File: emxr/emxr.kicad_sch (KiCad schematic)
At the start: 13 parts, among them J101 POWER, J103 Bus Conn, J104 GEQ_L_PRE, J105 GEQ_L_POST, J106 GEQ_R_PRE, J107 GEQ_R_POST, J108 AUDIO_OUT

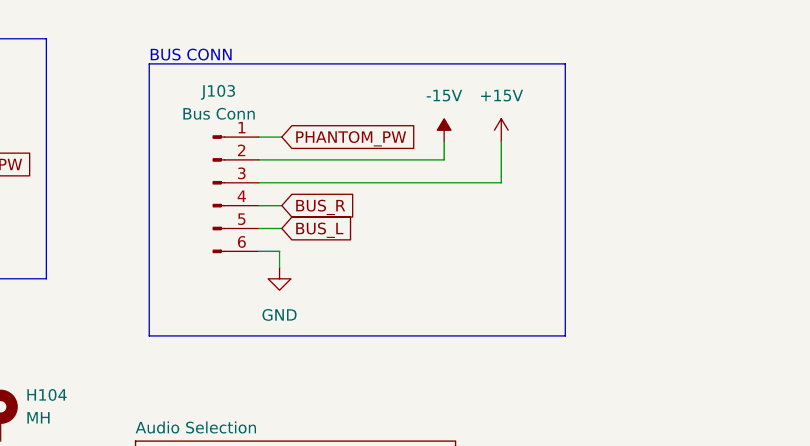
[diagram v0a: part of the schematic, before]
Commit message: finished pcb draft
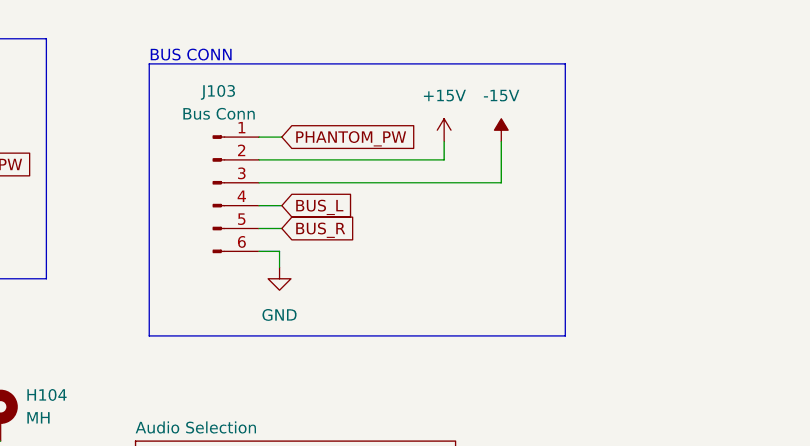
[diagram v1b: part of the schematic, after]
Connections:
- net +15V: now also J103.2 (Pin_2); no longer J103.3 (Pin_3)
- net -15V: now also J103.3 (Pin_3); no longer J103.2 (Pin_2)
- net BUS_L: now also J103.4 (Pin_4); no longer J103.5 (Pin_5)
- net BUS_R: now also J103.5 (Pin_5); no longer J103.4 (Pin_4)
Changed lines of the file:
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@@
+    )
+  )
+  (global_label "BUS_L" (shape input) (at 72.898 37.084 0) (fields_autoplaced)
+    (effects (font (size 1.27 1.27)) (justify left))
+    (property "Intersheet References" "${INTERSHEET_REFS}" (id 0) (at 81.1168 37.0046 0)
+      (effects (font (size 1.27 1.27)) (justify left) hide)
     )
   )
@@
     )
   )
-  (global_label "BUS_L" (shape input) (at 72.898 39.624 0) (fields_autoplaced)
-    (effects (font (size 1.27 1.27)) (justify left))
-    (property "Intersheet References" "${INTERSHEET_REFS}" (id 0) (at 81.1168 39.5446 0)
-      (effects (font (size 1.27 1.27)) (justify left) hide)
-    )
-  )
   (global_label "SINGAL_L_POST_GEQ" (shape input) (at 254.254 103.886 180) (fields_autoplaced)
     (effects (font (size 1.27 1.27)) (justify right))
@@
     )
   )
-  (global_label "BUS_R" (shape input) (at 72.898 37.084 0) (fields_autoplaced)
-    (effects (font (size 1.27 1.27)) (justify left))
-    (property "Intersheet References" "${INTERSHEET_REFS}" (id 0) (at 81.3587 37.0046 0)
-      (effects (font (size 1.27 1.27)) (justify left) hide)
-    )
-  )
   (global_label "SINGAL_R_PRE_GEQ" (shape input) (at 115.57 110.49 180) (fields_autoplaced)
     (effects (font (size 1.27 1.27)) (justify right))
@@
     )
   )
+  (global_label "BUS_R" (shape input) (at 72.898 39.624 0) (fields_autoplaced)
+    (effects (font (size 1.27 1.27)) (justify left))
+    (property "Intersheet References" "${INTERSHEET_REFS}" (id 0) (at 81.3587 39.5446 0)
+      (effects (font (size 1.27 1.27)) (justify left) hide)
+    )
+  )
   (symbol (lib_id "Connector:Conn_01x04_Male") (at 21.336 29.972 0) (unit 1)
     (in_bom yes) (on_board yes) (fields_autoplaced)
@@
     (pin "4")
   )
+  (symbol (lib_id "power:-15V") (at 97.282 29.972 0) (unit 1)
+    (in_bom yes) (on_board yes) (fields_autoplaced)
+    (property "Reference" "#PWR0117" (id 0) (at 97.282 27.432 0)
+      (effects (font (size 1.27 1.27)) hide)
+    )
+    (property "Value" "-15V" (id 1) (at 97.282 24.892 0))
+    (property "Footprint" "" (id 2) (at 97.282 29.972 0)
+      (effects (font (size 1.27 1.27)) hide)
+    )
+    (property "Datasheet" "" (id 3) (at 97.282 29.972 0)
+      (effects (font (size 1.27 1.27)) hide)
+    )
+    (pin "1")
+  )
   (symbol (lib_id "Mechanical:MountingHole_Pad") (at 34.036 60.706 0) (unit 1)
     (in_bom yes) (on_board yes) (fields_autoplaced)
@@
     (pin "1")
     (pin "2")
-  )
-  (symbol (lib_id "power:-15V") (at 36.576 26.162 0) (unit 1)
-    (in_bom yes) (on_board yes) (fields_autoplaced)
-    (property "Reference" "#PWR0102" (id 0) (at 36.576 23.622 0)
-      (effects (font (size 1.27 1.27)) hide)
-    )
-    (property "Value" "-15V" (id 1) (at 36.576 21.082 0))
-    (property "Footprint" "" (id 2) (at 36.576 26.162 0)
-      (effects (font (size 1.27 1.27)) hide)
-    )
-    (property "Datasheet" "" (id 3) (at 36.576 26.162 0)
-      (effects (font (size 1.27 1.27)) hide)
-    )
-    (pin "1")
   )
   (symbol (lib_id "power:GND") (at 28.956 37.592 0) (unit 1)
@@
     (pin "2")
   )
+  (symbol (lib_id "power:-15V") (at 36.576 26.162 0) (unit 1)
+    (in_bom yes) (on_board yes) (fields_autoplaced)
+    (property "Reference" "#PWR0102" (id 0) (at 36.576 23.622 0)
+      (effects (font (size 1.27 1.27)) hide)
+    )
+    (property "Value" "-15V" (id 1) (at 36.576 21.082 0))
+    (property "Footprint" "" (id 2) (at 36.576 26.162 0)
+      (effects (font (size 1.27 1.27)) hide)
+    )
+    (property "Datasheet" "" (id 3) (at 36.576 26.162 0)
+      (effects (font (size 1.27 1.27)) hide)
+    )
+    (pin "1")
+  )
   (symbol (lib_id "power:GND") (at 115.57 102.87 0) (unit 1)
     (in_bom yes) (on_board yes)
@@
     (pin "1")
   )
-  (symbol (lib_id "power:-15V") (at 90.932 29.972 0) (unit 1)
-    (in_bom yes) (on_board yes) (fields_autoplaced)
-    (property "Reference" "#PWR0117" (id 0) (at 90.932 27.432 0)
-      (effects (font (size 1.27 1.27)) hide)
-    )
-    (property "Value" "-15V" (id 1) (at 90.932 24.892 0))
-    (property "Footprint" "" (id 2) (at 90.932 29.972 0)
-      (effects (font (size 1.27 1.27)) hide)
-    )
-    (property "Datasheet" "" (id 3) (at 90.932 29.972 0)
+  (symbol (lib_id "power:+15V") (at 30.226 26.162 0) (unit 1)
+    (in_bom yes) (on_board yes) (fields_autoplaced)
+    (property "Reference" "#PWR0101" (id 0) (at 30.226 29.972 0)
+      (effects (font (size 1.27 1.27)) hide)
+    )
+    (property "Value" "+15V" (id 1) (at 30.226 21.082 0))
+    (property "Footprint" "" (id 2) (at 30.226 26.162 0)
+      (effects (font (size 1.27 1.27)) hide)
+    )
+    (property "Datasheet" "" (id 3) (at 30.226 26.162 0)
       (effects (font (size 1.27 1.27)) hide)
     )
@@
     (pin "3")
   )
+  (symbol (lib_id "power:+15V") (at 90.932 29.972 0) (unit 1)
+    (in_bom yes) (on_board yes)
+    (property "Reference" "#PWR0105" (id 0) (at 90.932 33.782 0)
+      (effects (font (size 1.27 1.27)) hide)
+    )
+    (property "Value" "+15V" (id 1) (at 90.932 24.892 0))
+    (property "Footprint" "" (id 2) (at 90.932 29.972 0)
+      (effects (font (size 1.27 1.27)) hide)
+    )
+    (property "Datasheet" "" (id 3) (at 90.932 29.972 0)
+      (effects (font (size 1.27 1.27)) hide)
+    )
+    (pin "1")
+  )
   (symbol (lib_id "Mechanical:MountingHole_Pad") (at 18.542 60.706 0) (unit 1)
     (in_bom yes) (on_board yes) (fields_autoplaced)
@@
     )
     (property "Datasheet" "~" (id 3) (at 27.94 27.432 0)
-      (effects (font (size 1.27 1.27)) hide)
-    )
-    (pin "1")
-  )
-  (symbol (lib_id "power:+15V") (at 97.282 29.972 0) (unit 1)
-    (in_bom yes) (on_board yes)
-    (property "Reference" "#PWR0105" (id 0) (at 97.282 33.782 0)
-      (effects (font (size 1.27 1.27)) hide)
-    )
-    (property "Value" "+15V" (id 1) (at 97.282 24.892 0))
-    (property "Footprint" "" (id 2) (at 97.282 29.972 0)
-      (effects (font (size 1.27 1.27)) hide)
-    )
-    (property "Datasheet" "" (id 3) (at 97.282 29.972 0)
-      (effects (font (size 1.27 1.27)) hide)
-    )
-    (pin "1")
-  )
-  (symbol (lib_id "power:+15V") (at 30.226 26.162 0) (unit 1)
-    (in_bom yes) (on_board yes) (fields_autoplaced)
-    (property "Reference" "#PWR0101" (id 0) (at 30.226 29.972 0)
-      (effects (font (size 1.27 1.27)) hide)
-    )
-    (property "Value" "+15V" (id 1) (at 30.226 21.082 0))
-    (property "Footprint" "" (id 2) (at 30.226 26.162 0)
-      (effects (font (size 1.27 1.27)) hide)
-    )
-    (property "Datasheet" "" (id 3) (at 30.226 26.162 0)
       (effects (font (size 1.27 1.27)) hide)
     )
@@
       (reference "#FLG0302") (unit 1) (value "PWR_FLAG") (footprint "")
     )
-    (path "/f7fcb284-2c50-4899-a801-6bc09b570947"
+    (path "/ca94f7d8-1a2e-4977-bdda-6569c606eee3"
       (reference "#PWR0101") (unit 1) (value "+15V") (footprint "")
     )
-    (path "/318c314c-3085-4786-b774-c74338b7a2e5"
+    (path "/969dab04-7c43-4161-8376-eb4539bfe8f0"
       (reference "#PWR0102") (unit 1) (value "-15V") (footprint "")
     )
@@
       (reference "#PWR0104") (unit 1) (value "GND") (footprint "")
     )
-    (path "/ee4aa2f5-45df-4dae-abad-1cf46d567827"
+    (path "/daf14d0e-21df-46a4-877f-4f85481a5d4a"
       (reference "#PWR0105") (unit 1) (value "+15V") (footprint "")
     )
@@
       (reference "#PWR0116") (unit 1) (value "GND") (footprint "")
     )
-    (path "/d20691b9-17e8-4af0-b9bd-2f8e4c1bd205"
+    (path "/1290aab4-682e-4097-b981-7d63f0a8b5a2"
       (reference "#PWR0117") (unit 1) (value "-15V") (footprint "")
     )

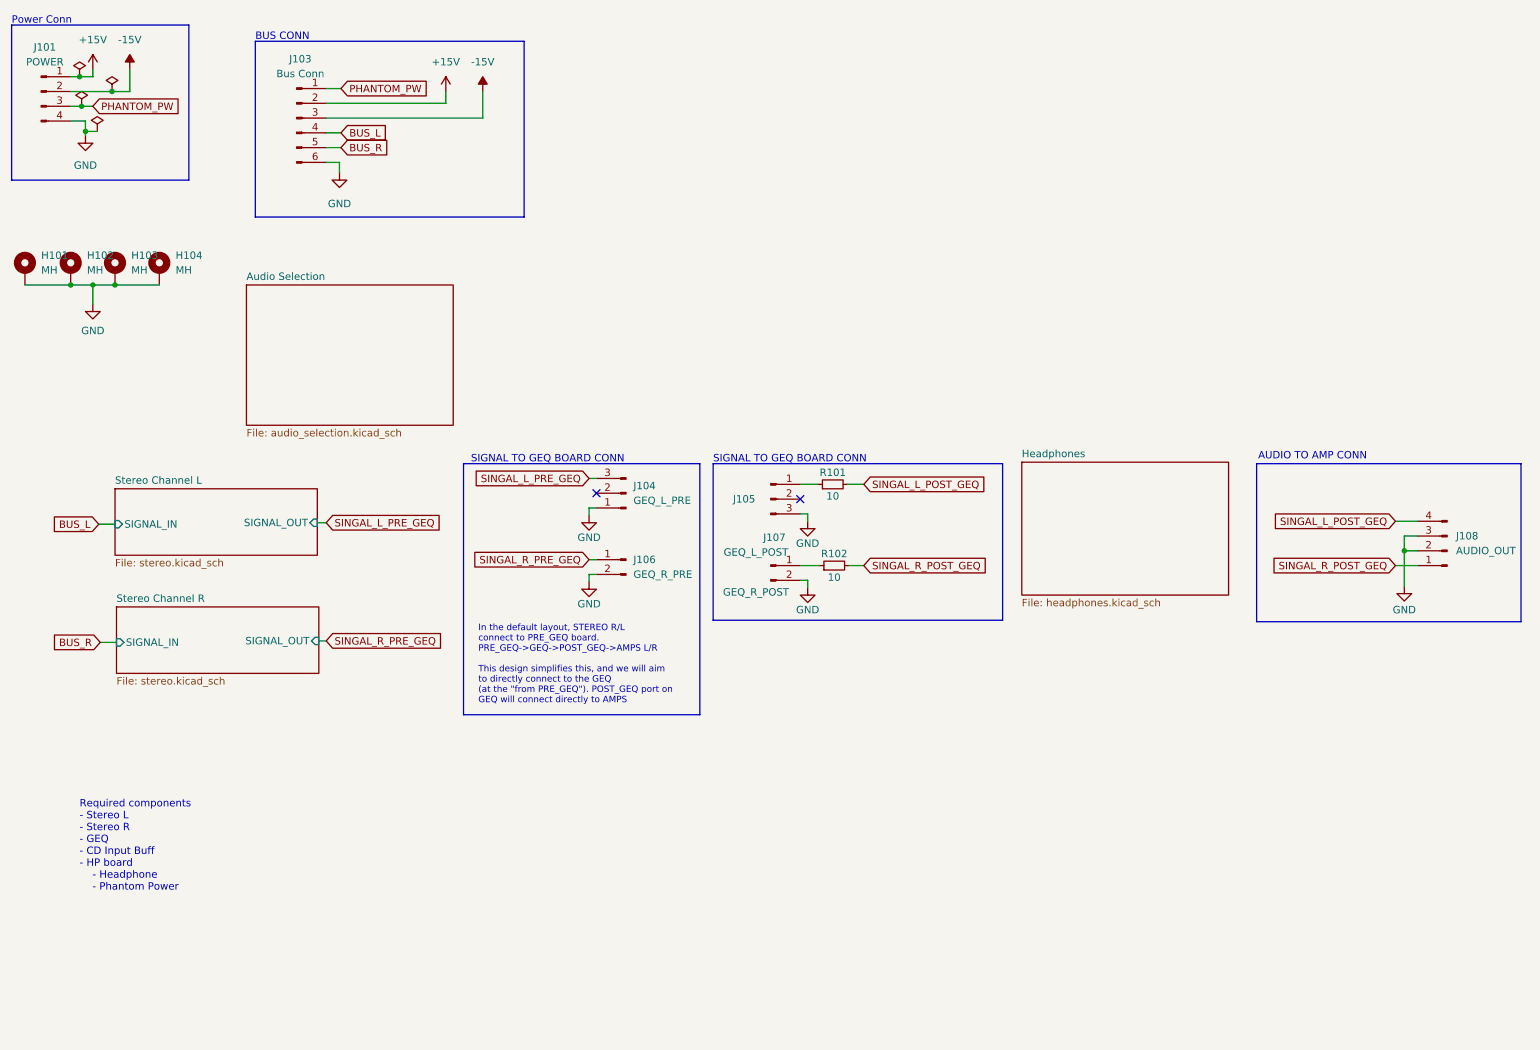
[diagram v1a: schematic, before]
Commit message: more cleaning up/finishing touches
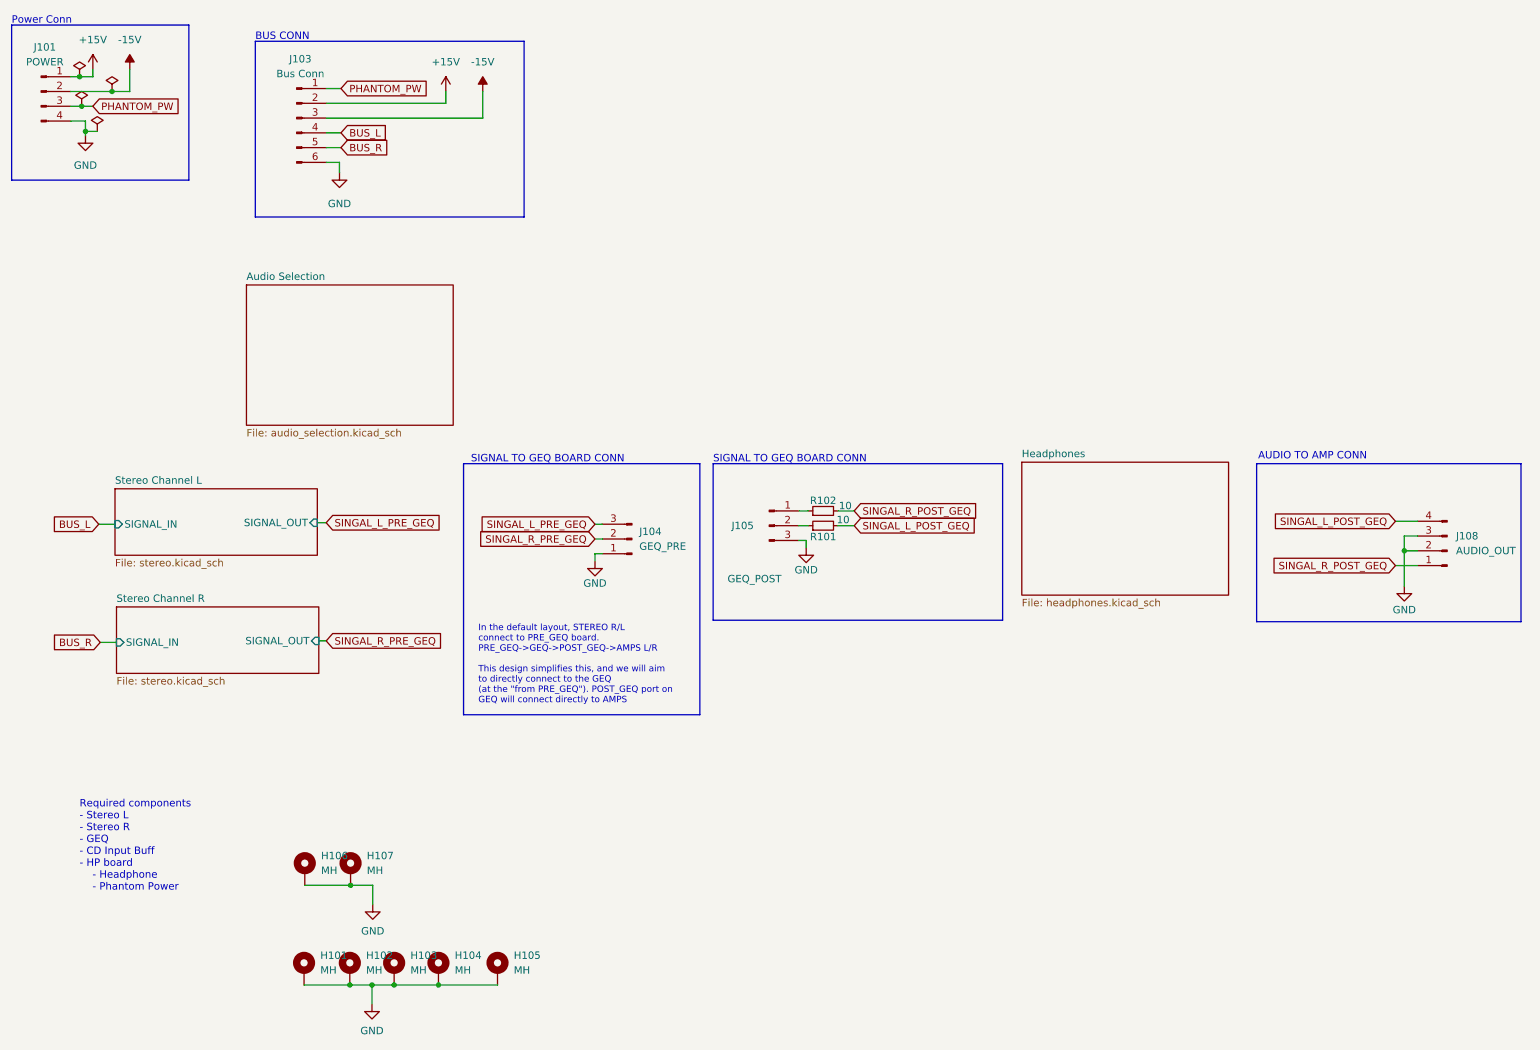
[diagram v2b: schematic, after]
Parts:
- removed J106: GEQ_R_PRE, Connector_JST:JST_XH_B2B-XH-A_1x02_P2.50mm_Vertical, symbol Connector:Conn_01x02_Male
- removed J107: GEQ_R_POST, Connector_JST:JST_XH_B2B-XH-A_1x02_P2.50mm_Vertical, symbol Connector:Conn_01x02_Male
- added H105, H106, H107: MH, MountingHole:MountingHole_3.2mm_M3_DIN965_Pad_TopBottom, symbol Mechanical:MountingHole_Pad
- J104: value GEQ_L_PRE -> GEQ_PRE
- J105: value GEQ_L_POST -> GEQ_POST
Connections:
- net GND: now also H105.1, H106.1, H107.1
- net SINGAL_R_PRE_GEQ: now also J104.2 (Pin_2)
- net at R101.1: now also J105.2 (Pin_2); no longer J105.1 (Pin_1)
- net at R102.1: now also J105.1 (Pin_1)
- no-connect marks 2 -> 0
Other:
- moved on the sheet: H101, H102, H103, H104, J104, J105, R101, R102
